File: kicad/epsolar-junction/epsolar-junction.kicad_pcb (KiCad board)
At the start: 2 copper layers, 87.6 x 50.8 mm, 22 parts, among them J1 Conn_01x02, J10 EDG, J11 DISPLAY, J12 I2C, J13 USB_B_Micro, J14 USBSERIAL, J2 Conn_01x02, J3 Conn_01x02, J4 Conn_01x02, J5 Conn_01x02, J6 Conn_01x08, J7 Conn_01x08, J8 Conn_01x02, J9 RJ45, SW1 SW_Push, SW2 SW_Push

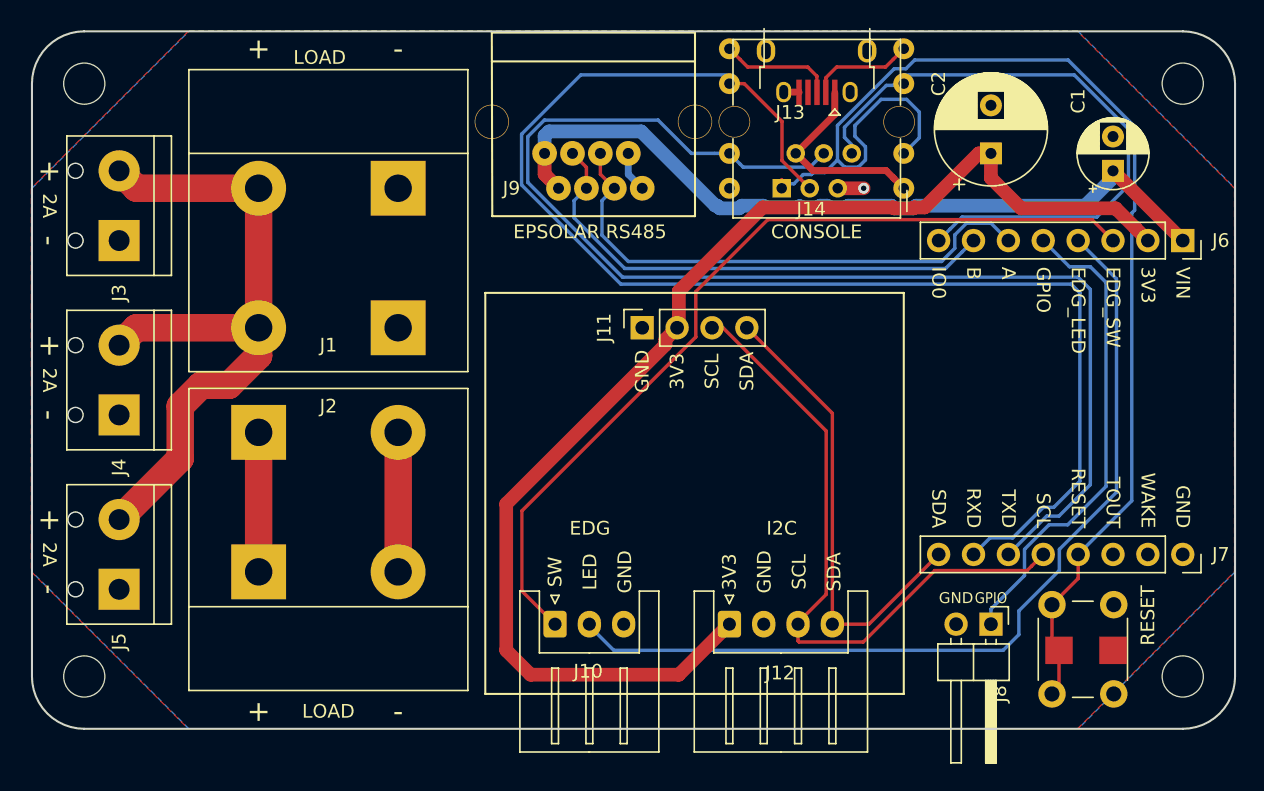
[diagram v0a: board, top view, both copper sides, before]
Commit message: PCBs update
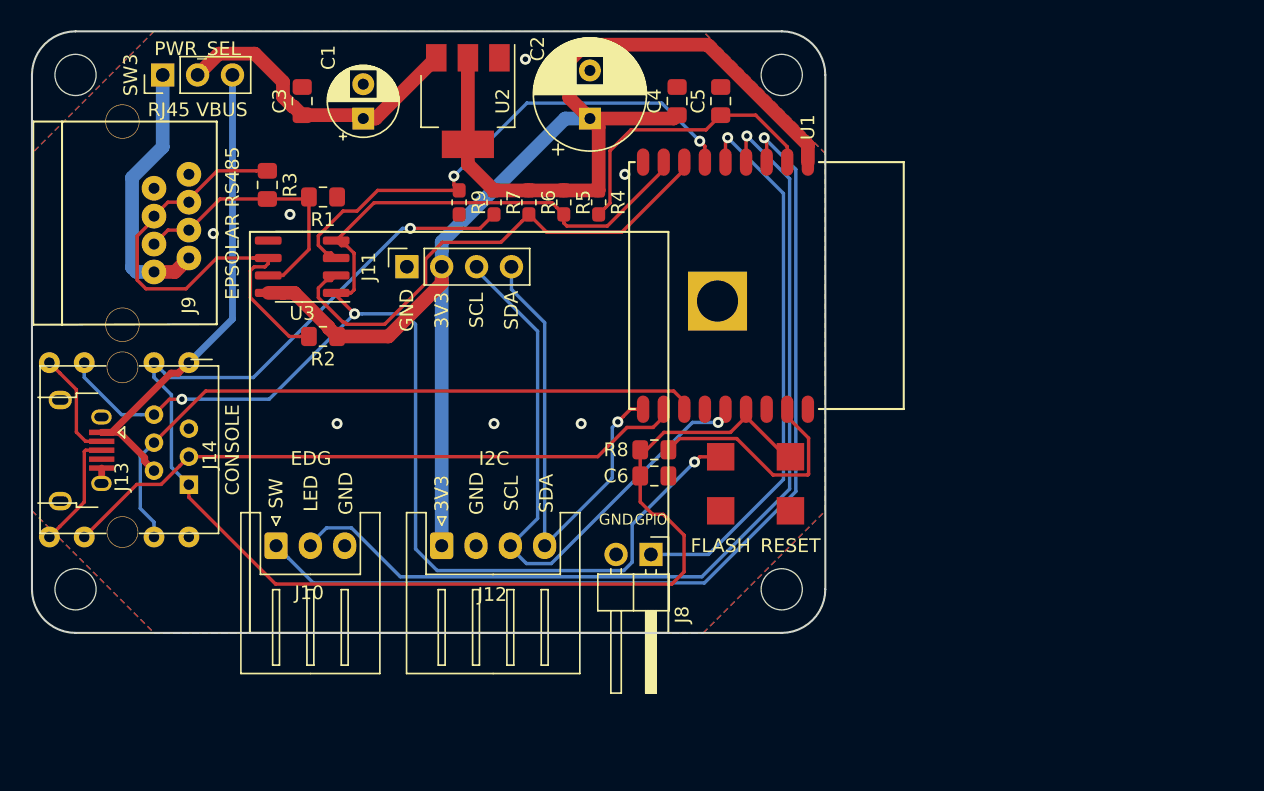
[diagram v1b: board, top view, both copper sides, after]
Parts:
- removed J1, J2: Conn_01x02, lib:TerminalBlock_P10.16mm
- removed J3, J4, J5: Conn_01x02, TerminalBlock:TerminalBlock_bornier-2_P5.08mm
- removed J6, J7: Conn_01x08, Connector_PinSocket_2.54mm:PinSocket_1x08_P2.54mm_Vertical
- added C3: 0.1uF, Capacitor_SMD:C_0805_2012Metric_Pad1.15x1.40mm_HandSolder, F.Cu at (137.8, 90.2)
- added C4: 0.1uF, Capacitor_SMD:C_0805_2012Metric_Pad1.15x1.40mm_HandSolder, F.Cu at (165.1, 90.2)
- added C5: 0.1uF, Capacitor_SMD:C_0805_2012Metric_Pad1.15x1.40mm_HandSolder, F.Cu at (168.3, 90.2)
- added C6: 0.1uF, Capacitor_SMD:C_0805_2012Metric_Pad1.15x1.40mm_HandSolder, F.Cu at (163.4, 117.5)
- added R1: 20K, Resistor_SMD:R_0805_2012Metric_Pad1.15x1.40mm_HandSolder, F.Cu at (139.3, 97.2)
- added R2: 20K, Resistor_SMD:R_0805_2012Metric_Pad1.15x1.40mm_HandSolder, F.Cu at (139.3, 107.3)
- added R3: 200, Resistor_SMD:R_0805_2012Metric_Pad1.15x1.40mm_HandSolder, F.Cu at (135.3, 96.3)
- added R4: 10K, Resistor_SMD:R_0603_1608Metric_Pad1.05x0.95mm_HandSolder, F.Cu at (159.4, 97.5)
- added R5: 10K, Resistor_SMD:R_0603_1608Metric_Pad1.05x0.95mm_HandSolder, F.Cu at (156.8, 97.5)
- added R6: 10K, Resistor_SMD:R_0603_1608Metric_Pad1.05x0.95mm_HandSolder, F.Cu at (154.3, 97.5)
- added R7: 10K, Resistor_SMD:R_0603_1608Metric_Pad1.05x0.95mm_HandSolder, F.Cu at (151.8, 97.5)
- added R8: 470, Resistor_SMD:R_0805_2012Metric_Pad1.15x1.40mm_HandSolder, F.Cu at (163.4, 115.6)
- added R9: 10K, Resistor_SMD:R_0603_1608Metric_Pad1.05x0.95mm_HandSolder, F.Cu at (149.2, 97.5)
- added SW3: SW_SPDT, Connector_PinHeader_2.54mm:PinHeader_1x03_P2.54mm_Vertical, F.Cu at (127.6, 88.3)
- added U1: ESP-13-WROOM-02, lib:ESP-13-WROOM-02, F.Cu at (174.6, 94.6)
- added U2: AMS1117-3.3, Package_TO_SOT_SMD:SOT-223-3_TabPin2, F.Cu at (149.9, 90.2)
- added U3: MAX3485, Package_SO:SOIC-8_3.9x4.9mm_P1.27mm, F.Cu at (137.8, 102.2)
- SW1: footprint Button_Switch_THT:SW_PUSH_6mm -> lib:tactile_switch_smd_4x3mm_2p
- moved J13 60.8 mm to (121.3, 115.6), turned to 270 degrees
- moved C1 54.7 mm to (142.2, 91.4)
- moved J14 48.3 mm to (129.5, 118.1), turned to 270 degrees
- moved J9 32.4 mm to (127.0, 99.1), turned to 270 degrees
- moved REF** 29.9 mm to (172.7, 125.7)
- moved C2 29.3 mm to (158.8, 91.4)
- moved SW2 29.3 mm to (168.3, 118.1), turned to 270 degrees
- moved REF** 29.2 mm to (172.7, 88.3)
- moved J8 25.3 mm to (163.2, 123.2)
- moved SW1 24.4 mm to (173.4, 118.1), turned to 270 degrees
- moved J12 21.7 mm to (148.0, 122.6)
- moved J10 21.1 mm to (135.9, 122.6)
- moved J11 17.7 mm to (145.4, 102.2)
- moved REF** 6.38 mm to (121.3, 125.7)
- moved REF** 0.90 mm to (121.3, 88.3)
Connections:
- J13 pad 4: (no net) -> Net-(J13-Pad4)
- J9 pad 1: /VIN -> /VCTRLR
- J9 pad 2: /VIN -> /VCTRLR
- SW2 pad 1: /RESET -> /IO0
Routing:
- net /IO0: track 45.0 -> 110.1 mm, vias 0 -> 3
- net /RXD: track 98.9 -> 46.4 mm
- net /LOADPLUS: track 50.9 -> 0.00 mm
- net /TXD: track 93.7 -> 48.8 mm
- net /IO15: track 0.00 -> 38.1 mm, vias 0 -> 2
- net /IO2: track 0.00 -> 37.2 mm
- net /VIN: track 57.1 -> 22.5 mm
- net /VBUS: track 14.5 -> 35.8 mm
- net /EN: track 0.00 -> 21.0 mm
- net /VCTRLR: track 0.00 -> 19.6 mm
- net /3V3: track 91.9 -> 110.4 mm
- net /WAKE: track 0.00 -> 17.0 mm
- net /B: track 36.9 -> 20.3 mm
- net /RESET: track 92.9 -> 104.4 mm, vias 0 -> 1
- net Net-(J2-Pad2): track 10.2 -> 0.00 mm
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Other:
- board size 87.6 x 50.8 mm -> 57.8 x 43.8 mm
- board text added: "FLASH"
- board text added: "PWR_SEL"
- board text added: "RJ45 VBUS"
- board text removed: "+"
- board text removed: "-"
- board text removed: "2A"
- board text removed: "A"
- board text removed: "B"
- board text removed: "EDG_LED"
- board text removed: "EDG_SW"
- board text removed: "IO0"
- board text removed: "LOAD"
- board text removed: "RXD"
- board text removed: "TOUT"
- board text removed: "TXD"
- board text removed: "VIN"
- board text removed: "WAKE"
